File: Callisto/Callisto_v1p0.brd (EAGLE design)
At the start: 160 x 120 mm, 93 parts, among them J1 20-pos, J10 RJ45_TH_VERT, J11 RJ45_TH_VERT, J12 10-pos, J13 RJ45_TH_VERT, J14 RJ45_TH_VERT, J15 RJ45_TH_VERT, J16 RJ45_TH_VERT, J17 RJ45_TH_VERT, J18 RJ45_TH_VERT, J19 RJ45_TH_VERT, J2 2-pos, J20 RJ45_TH_VERT, J21 RJ45_TH_VERT, J22 RJ45_TH_VERT, J23 RJ45_TH_VERT, J24 RJ45_TH_VERT, J25 RJ45_TH_VERT, J3 2-pos, J4 4-pos, J5 RJ45_TH_VERT, J6 RJ45_TH_VERT, J7 RJ45_TH_VERT, J8 RJ45_TH_VERT, J9 RJ45_TH_VERT, U3 AD8495ARMZ, U6 AD8495ARMZ

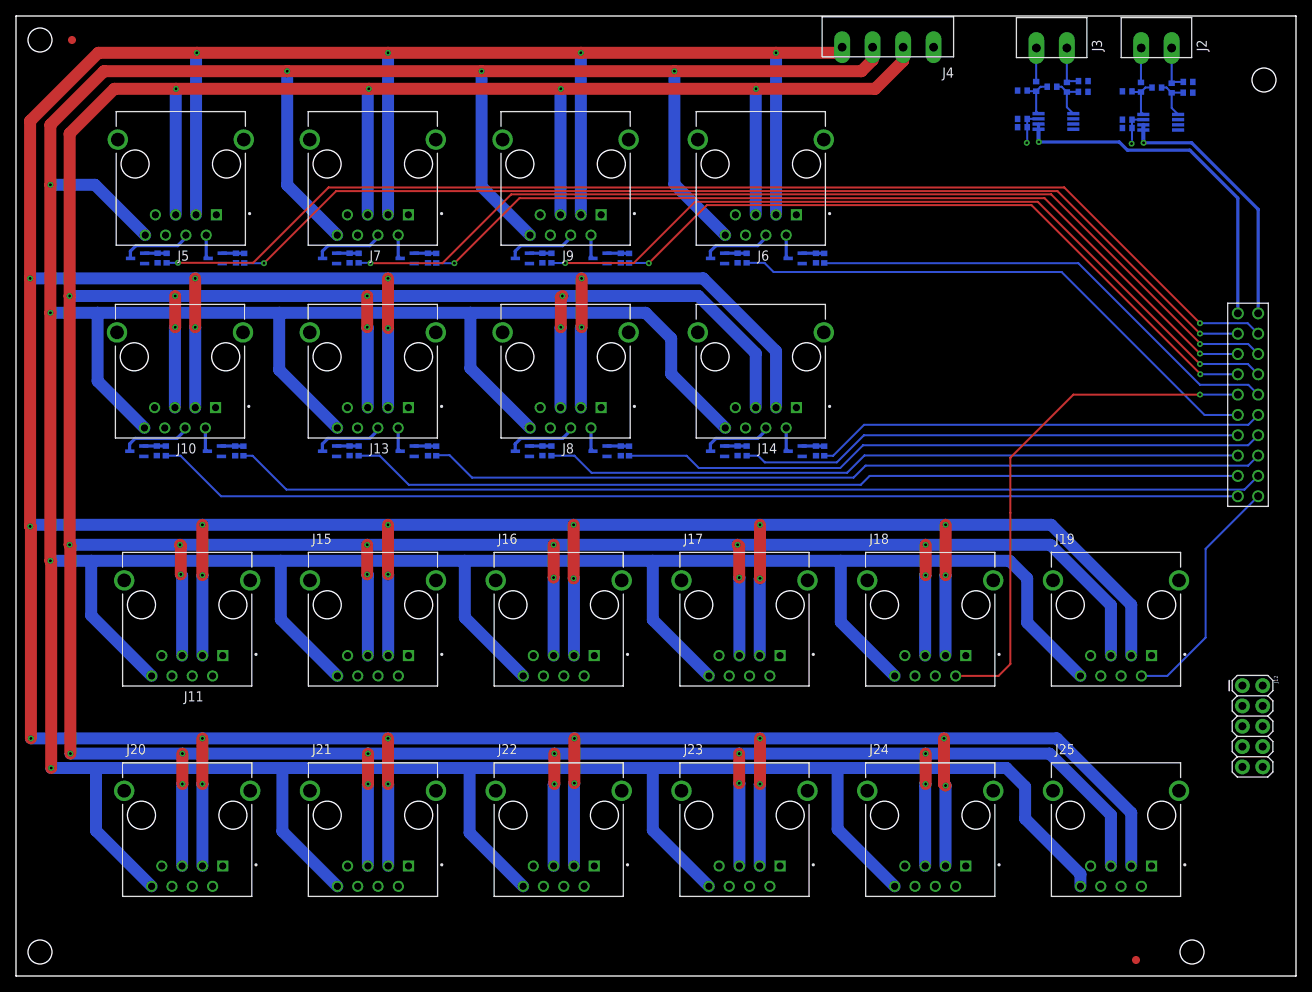
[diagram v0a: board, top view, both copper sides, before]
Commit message: Updated Board
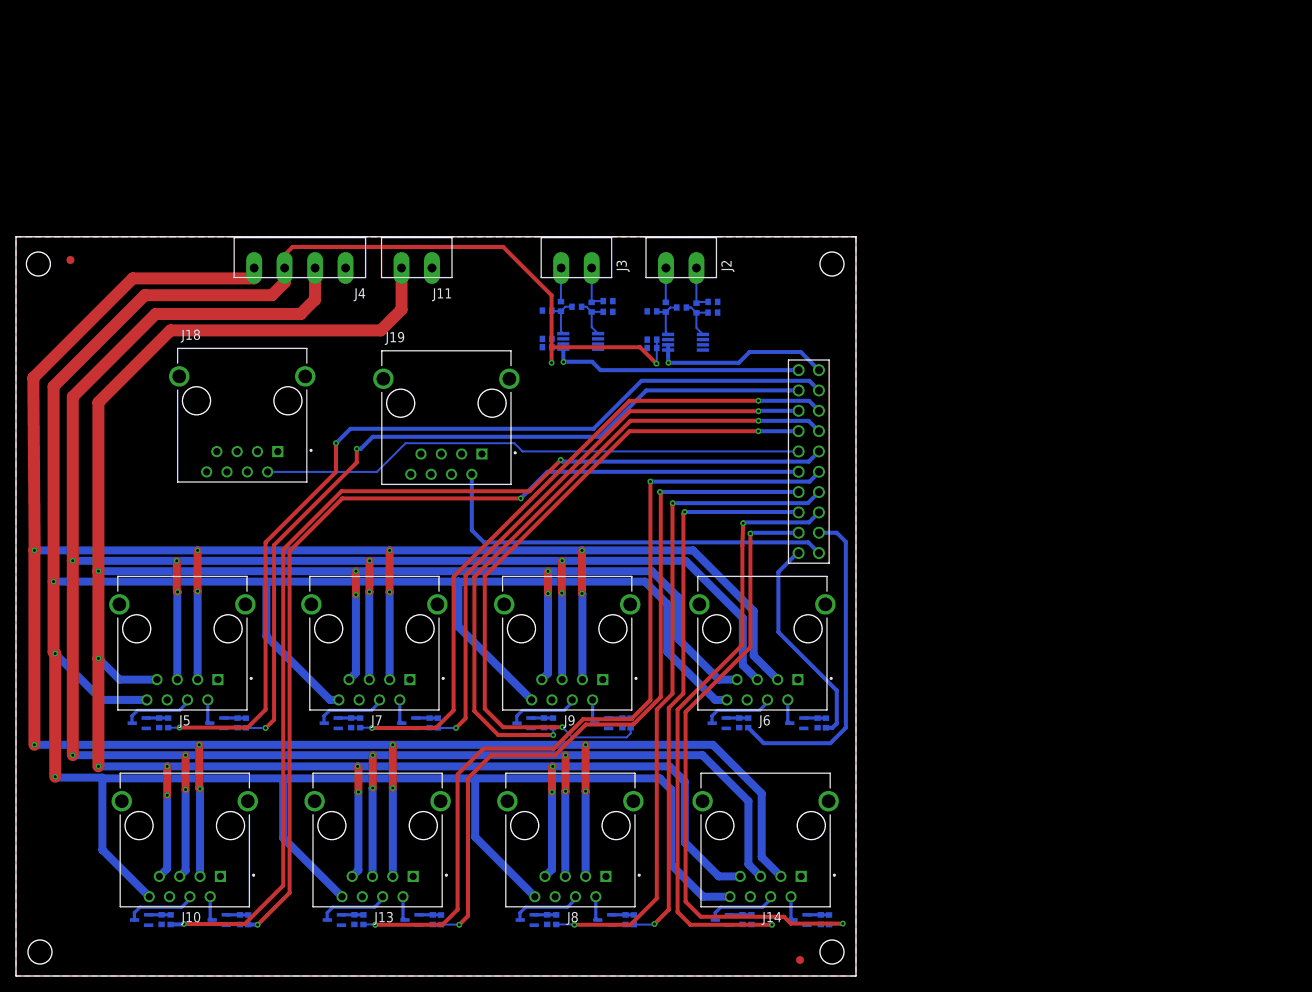
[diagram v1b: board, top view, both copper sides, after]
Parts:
- removed J12: 10-pos, 3D_MIG_Controller:2X5
- removed J15, J16, J17, J20, J21, J22, J23, J24, J25: RJ45_TH_VERT, 3D_MIG_Controller:ASSMANN_A-2014-2S-4-N-R
- J11: value RJ45_TH_VERT -> 2-pos; device 3D_MIG_Controller:ASSMANN_A-2014-2S-4-N-R -> 3D_MIG_Controller:2_3.81MM_PITCH
- moved J18 89.7 mm to (28.3, 71.9)
- moved J19 87.4 mm to (53.8, 71.6)
- moved J4 78.5 mm to (41.2, 88.5)
- moved J3 65.5 mm to (72.0, 88.5)
- moved R121 65.5 mm to (72.0, 83.6)
- moved 130 65.5 mm to (81.2, 83.6)
- moved C12 65.5 mm to (87.1, 82.9)
- moved C13 65.5 mm to (79.5, 83.1)
- moved C14 65.5 mm to (79.5, 79.5)
- moved C15 65.5 mm to (79.5, 78.5)
- moved C6 65.5 mm to (70.1, 83.7)
- moved C7 65.5 mm to (74.0, 83.0)
- moved J2 65.5 mm to (85.1, 88.5)
- moved R131 65.5 mm to (85.1, 83.5)
- moved U3 65.5 mm to (70.6, 79.3)
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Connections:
- removed net IO_SIGNAL: J11.2, J15.2, J16.2, J17.2, J20.2, J21.2, J22.2, J23.2, J24.2, J25.2
- removed net P2_03: J12.1
- removed net P2_04: J12.3
- removed net P2_05: J12.5
- removed net P2_06: J12.7
- removed net P2_07: J12.9
- removed net VDD+: C10.P$1, C14.P$1, C15.P$1, C9.P$1, U3.7, U6.7
- net GND: now also J11.P$1; no longer J11.1, J11.4, J11.6, J12.10, J12.2, J12.4, J12.6, J12.8, J15.1, J15.4, J15.6, J16.1, J16.4, J16.6, J17.1, J17.4, J17.6, J20.1, J20.4, J20.6, J21.1, J21.4, J21.6, J22.1, J22.4, J22.6, J23.1, J23.4, J23.6, J24.1, J24.4, J24.6, J25.1, J25.4, J25.6
- net P4_09: now also R9.P$1; no longer R26.P$1
- net P4_10: now also R10.P$1; no longer R25.P$1
- net P4_11: now also R37.P$1; no longer R34.P$1
- net P4_12: now also R38.P$1; no longer R33.P$1
- net P4_13: now also R17.P$1; no longer R18.P$1
- net P4_14: now also R18.P$1; no longer R17.P$1
- net P4_15: now also R33.P$1; no longer R38.P$1
- net P7_06: now also R26.P$1; no longer R9.P$1
- net P7_07: now also R25.P$1; no longer R10.P$1
- net PB_00: now also R34.P$1; no longer R37.P$1
- net VDD: no longer J11.5, J15.5, J16.5, J17.5, J20.5, J21.5, J22.5, J23.5, J24.5, J25.5
- net VDD-12: now also J11.P$2; no longer J11.7, J15.7, J16.7, J17.7, J20.7, J21.7, J22.7, J23.7, J24.7, J25.7
- net VDD12: no longer J11.3, J15.3, J16.3, J17.3, J20.3, J21.3, J22.3, J23.3, J24.3, J25.3
- net VDD5: now also C10.P$1, C14.P$1, C15.P$1, C9.P$1, U3.7, U6.7; no longer J11.8, J15.8, J16.8, J17.8, J20.8, J21.8, J22.8, J23.8, J24.8, J25.8
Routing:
- net VDD12: track 874.1 -> 385.5 mm, vias 33 -> 14
- net VDD: track 806.9 -> 366.4 mm, vias 33 -> 14
- net VDD5: track 867.7 -> 445.8 mm, vias 7 -> 5
- net VDD-12: track 0.00 -> 350.9 mm, vias 0 -> 13
- net P4_09: track 136.1 -> 27.1 mm
- net P4_10: track 129.3 -> 40.9 mm
- net P7_06: track 61.1 -> 130.3 mm, vias 0 -> 2
- net PB_00: track 56.4 -> 106.3 mm, vias 0 -> 2
- net P7_07: track 69.3 -> 117.3 mm, vias 0 -> 2
- net P5_11: track 124.3 -> 84.6 mm
- net P5_12: track 111.6 -> 72.0 mm
- net P8_05: track 135.3 -> 100.4 mm
- net P4_11: track 111.9 -> 78.1 mm, vias 0 -> 2
- net P5_13: track 147.9 -> 114.2 mm
- net P4_15: track 63.2 -> 92.4 mm, vias 0 -> 2
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- added copper zone on layer 1, net GND
- added copper zone on layer 16, net GND
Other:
- board size 160 x 120 mm -> 105 x 92.4 mm
